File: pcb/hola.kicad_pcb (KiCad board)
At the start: 2 copper layers, 60 x 49 mm, 39 parts, among them J1 USB_B, J2 USB_B_Micro, J3 Conn_01x08, J4 Conn_01x02, Q1 DTB123T, U1 TPS61090, U2 MCP73871

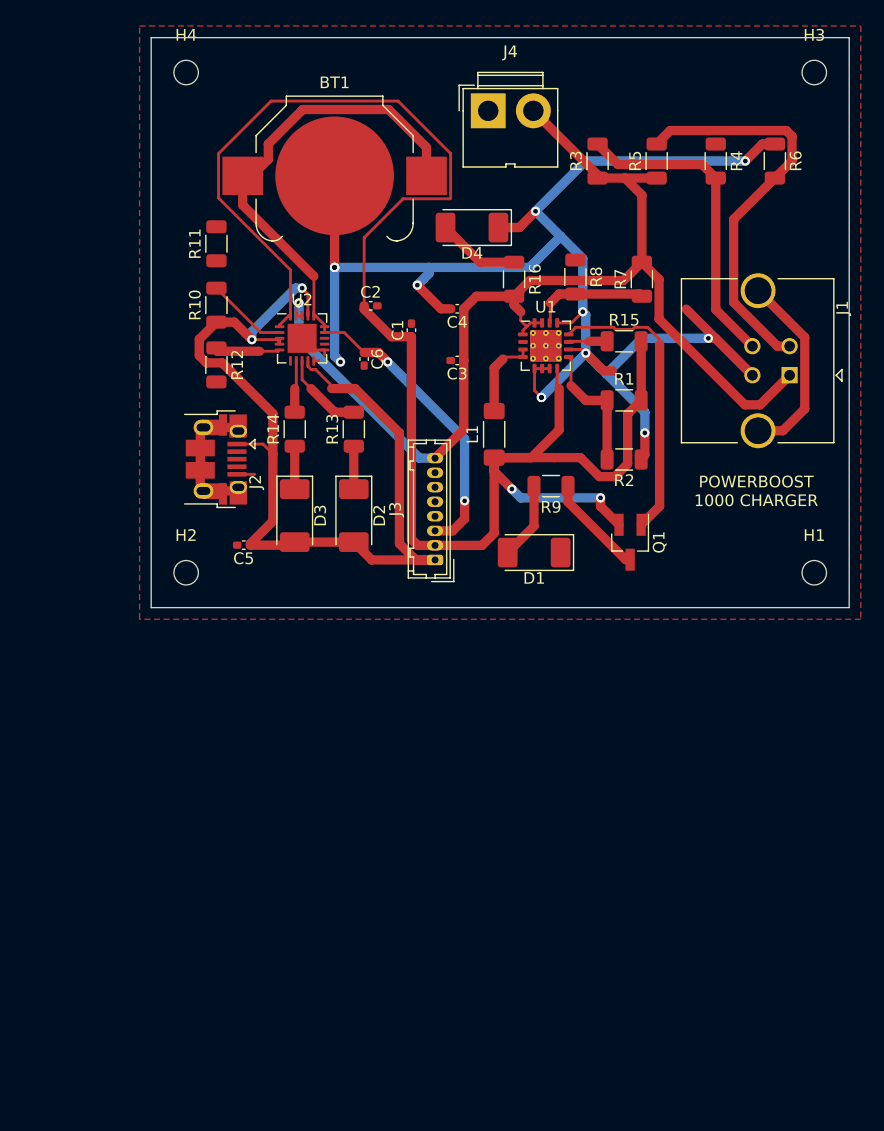
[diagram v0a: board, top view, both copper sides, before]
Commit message: actualizacion
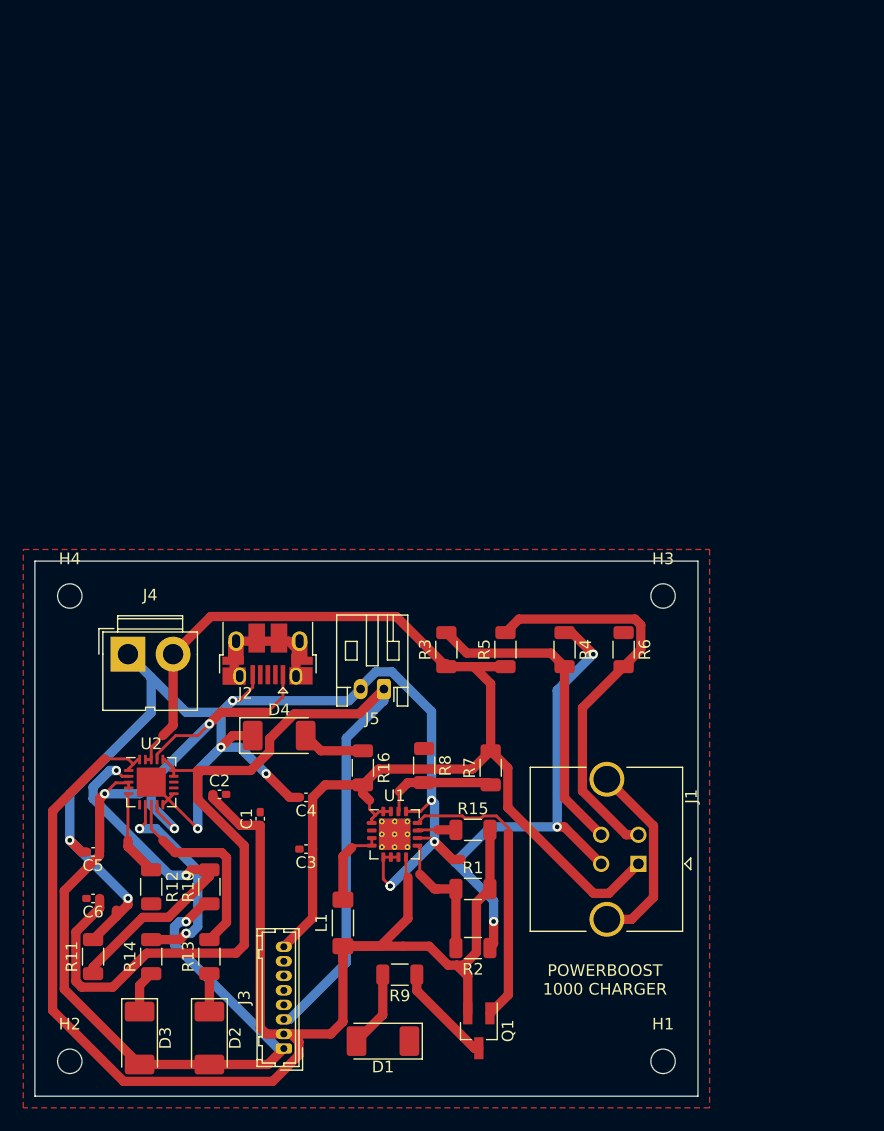
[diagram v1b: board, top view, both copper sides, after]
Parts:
- removed BT1: Battery_Cell, Battery:BatteryHolder_Keystone_3000_1x12mm
- added J5: Conn_01x02, Connector_JST:JST_PH_S2B-PH-K_1x02_P2.00mm_Horizontal, F.Cu at (148.0, 100.0)
- moved R11 62.2 mm to (123.0, 123.0)
- moved J4 56.0 mm to (126.0, 97.0)
- moved C6 51.9 mm to (123.0, 118.0), turned to 180 degrees
- moved R10 50.0 mm to (133.0, 117.0)
- moved R13 47.0 mm to (133.0, 123.0)
- moved R14 47.0 mm to (128.0, 123.0)
- moved D3 46.8 mm to (127.0, 130.0)
- moved H3 46.8 mm to (172.0, 92.0)
- moved D4 46.7 mm to (139.0, 104.0), turned to 0 degrees
- moved D2 46.6 mm to (133.0, 130.0)
- moved H4 46.1 mm to (121.0, 92.0)
- moved R12 45.2 mm to (128.0, 117.0)
- moved C1 44.0 mm to (137.4, 111.1)
- moved C2 44.0 mm to (133.9, 109.1)
- moved C3 44.0 mm to (141.3, 113.8)
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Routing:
- net +VSW: track 64.9 -> 96.6 mm, vias 2 -> 0
- net GND: track 142.2 -> 169.0 mm
- net Net-(R10-Pad2): track 7.01 -> 32.1 mm, vias 0 -> 2
- net +BATT: track 148.8 -> 135.0 mm, vias 2 -> 0
- net Net-(R14-Pad2): track 4.66 -> 18.0 mm, vias 0 -> 2
- net VBUS: track 84.3 -> 95.7 mm, vias 2 -> 4
- net Net-(R13-Pad2): track 8.10 -> 17.2 mm
- net +5V: track 99.5 -> 107.8 mm, vias 1 -> 0
- net Net-(R12-Pad1): track 5.71 -> 7.39 mm
- net Net-(D4-Pad2): track 7.13 -> 5.46 mm
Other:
- board size 60 x 49 mm -> 57 x 46 mm
- board text added: "Dimension: 57mm x 46mm Minimos (Frabricante): 10 mils Grillas: 1mm via:1.2mm / 0.8mm margen: 1mm pista: 0.8mm / 0.25mm distancia de borde: 1mm relleno capa frontal: GND esto ya que se tenia varios componentes SMD que compartian GND en la capa frontal"
- board text removed: "Minimos (Frabricante): 10 mils Grillas: 1mm 0.5 via:1.2mm / 0.8mm margen: 0.5mm pista: 1.2mm /1mm / 0.8mm distancia de borde: 0.5mm terminacion: a determinar"

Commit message: actualizacion
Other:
- board text added: "Dimension: 57mm x 46mm Minimos (Frabricante): 10 mils Grillas: 1mm via: 0.8mm / 0.4mm margen: 1mm pista: 0.8mm / 0.25mm distancia de borde: 1mm relleno capa frontal: GND esto ya que se tenia varios componentes SMD que compartian GND en la capa frontal"
- board text removed: "Dimension: 57mm x 46mm Minimos (Frabricante): 10 mils Grillas: 1mm via:1.2mm / 0.8mm margen: 1mm pista: 0.8mm / 0.25mm distancia de borde: 1mm relleno capa frontal: GND esto ya que se tenia varios componentes SMD que compartian GND en la capa frontal"
